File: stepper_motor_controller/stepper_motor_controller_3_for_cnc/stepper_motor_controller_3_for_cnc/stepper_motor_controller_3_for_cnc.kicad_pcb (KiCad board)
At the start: 2 copper layers, 119.4 x 45.7 mm, 44 parts, among them J2 178-009-613R571, U1 74LS74, U11 LM317_TO-220, U3 74LS136

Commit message: centering pcb above origin not below
centering pcb above origin not below
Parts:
- moved R38 144.5 mm to (96.6, -29.9)
- moved R39 144.5 mm to (75.0, -28.6)
- moved R5 144.5 mm to (64.8, -28.6)
- moved R70 144.5 mm to (64.8, -3.23)
- moved R72 144.5 mm to (75.0, -3.23)
- moved U10 144.5 mm to (54.7, -7.05)
- moved U9 144.5 mm to (62.3, -24.8)
- moved J2 144.5 mm to (121.9, -15.9)
- moved R17 144.5 mm to (101.7, -18.5)
- moved R18 144.5 mm to (89.0, -21.0)
- moved R37 144.5 mm to (91.5, -27.4)
- moved R44 144.5 mm to (42.0, -28.6)
- moved R47 144.5 mm to (24.2, -28.4)
- moved R49 144.5 mm to (31.8, -3.23)
- moved R60 144.5 mm to (31.8, -28.6)
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
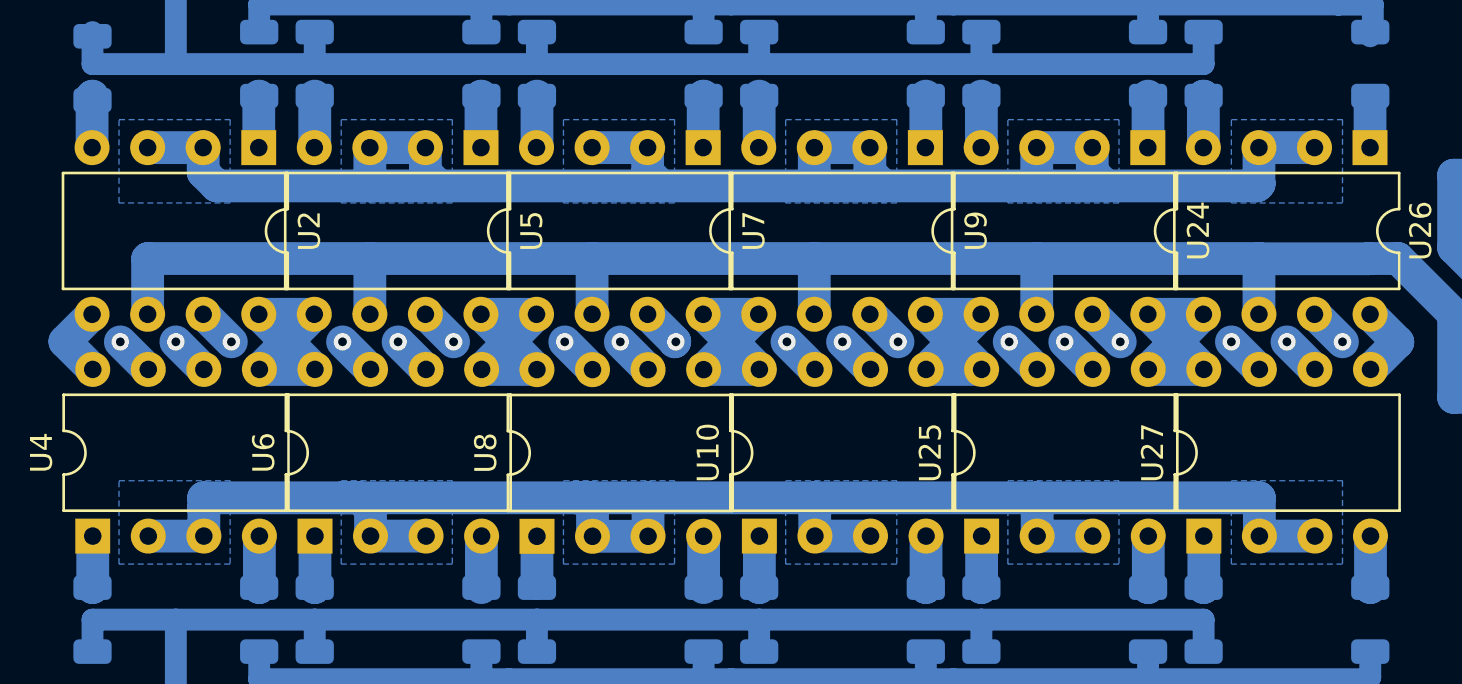
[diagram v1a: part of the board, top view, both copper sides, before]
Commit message: pcb errors
pcb errors
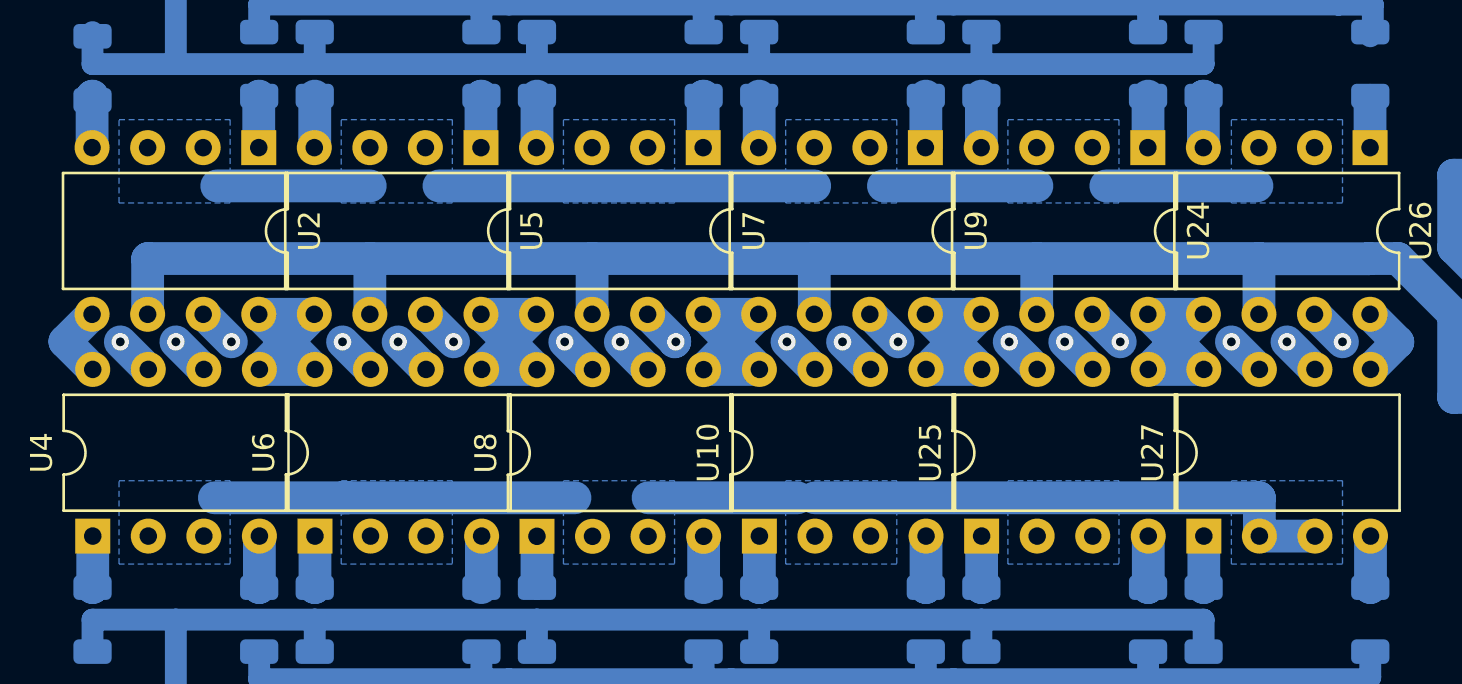
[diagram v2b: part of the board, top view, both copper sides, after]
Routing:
- net VCC: track 207.9 -> 136.8 mm
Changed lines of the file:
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@@
   (segment (start 49.5938 -14.66) (end 48.3238 -15.93) (width 1.5) (layer "B.Cu") (net 16))
   (via (at 99.9338 -35.11) (size 3) (drill 2.4) (layers "F.Cu" "B.Cu") (free) (net 17))
-  (segment (start 49.5938 -7.04) (end 47.0538 -7.04) (width 1.5) (layer "B.Cu") (net 17))
   (segment (start 124.5488 -26.065) (end 114.3888 -26.065) (width 0.5) (layer "B.Cu") (net 17))
-  (segment (start 49.5938 -8.8) (end 57.2138 -8.8) (width 1.5) (layer "B.Cu") (net 17))
-  (segment (start 46.2538 -8.8) (end 49.5938 -8.8) (width 1.5) (layer "B.Cu") (net 17))
   (segment (start 104.8388 -29.9) (end 104.8388 -30.205) (width 1.5) (layer "B.Cu") (net 17))
   (segment (start 127.2938 -18.7) (end 128.3338 -19.74) (width 0.5) (layer "B.Cu") (net 17))
-  (segment (start 47.0338 -24.81) (end 49.5738 -24.81) (width 1.5) (layer "B.Cu") (net 17))
-  (segment (start 77.5338 -23.160382) (end 77.433418 -23.06) (width 1.5) (layer "B.Cu") (net 17))
-  (segment (start 67.3738 -8.8) (end 67.3838 -8.79) (width 1.5) (layer "B.Cu") (net 17))
   (segment (start 77.5338 -8.8) (end 77.5438 -8.79) (width 1.5) (layer "B.Cu") (net 17))
-  (segment (start 57.1938 -24.81) (end 59.7338 -24.81) (width 1.5) (layer "B.Cu") (net 17))
-  (segment (start 36.8738 -23.08) (end 36.8938 -23.06) (width 1.5) (layer "B.Cu") (net 17))
-  (segment (start 40.03243 -23.06) (end 39.4138 -23.67863) (width 1.5) (layer "B.Cu") (net 17))
-  (segment (start 39.4438 -7.05) (end 36.9038 -7.05) (width 1.5) (layer "B.Cu") (net 17))
-  (segment (start 77.5238 -23.170382) (end 77.5338 -23.160382) (width 1.5) (layer "B.Cu") (net 17))
-  (segment (start 36.8738 -24.81) (end 39.4138 -24.81) (width 1.5) (layer "B.Cu") (net 17))
-  (segment (start 26.7138 -24.81) (end 29.2538 -24.81) (width 1.5) (layer "B.Cu") (net 17))
-  (segment (start 39.4138 -23.67863) (end 39.4138 -24.81) (width 1.5) (layer "B.Cu") (net 17))
-  (segment (start 29.2738 -8.31) (end 29.2738 -8.8) (width 1.5) (layer "B.Cu") (net 17))
-  (segment (start 67.3638 -23.07) (end 67.3738 -23.06) (width 1.5) (layer "B.Cu") (net 17))
-  (segment (start 36.4038 -8.8) (end 36.9038 -8.3) (width 1.5) (layer "B.Cu") (net 17))
-  (segment (start 49.5938 -7.04) (end 49.5938 -8.8) (width 1.5) (layer "B.Cu") (net 17))
+  (segment (start 35.6238 -8.8) (end 35.9138 -8.8) (width 1.5) (layer "B.Cu") (net 17))
+  (segment (start 29.7638 -8.8) (end 35.6238 -8.8) (width 1.5) (layer "B.Cu") (net 17))
   (segment (start 36.8938 -23.06) (end 29.87243 -23.06) (width 1.5) (layer "B.Cu") (net 17))
-  (segment (start 29.87243 -23.06) (end 29.2538 -23.67863) (width 1.5) (layer "B.Cu") (net 17))
-  (segment (start 59.7638 -7.05) (end 57.2238 -7.05) (width 1.5) (layer "B.Cu") (net 17))
   (segment (start 104.8388 -30.205) (end 99.9338 -35.11) (width 1.5) (layer "B.Cu") (net 17))
-  (segment (start 57.2138 -7.06) (end 57.2238 -7.05) (width 1.5) (layer "B.Cu") (net 17))
   (segment (start 77.5438 -8.79) (end 77.5438 -7.05) (width 1.5) (layer "B.Cu") (net 17))
-  (segment (start 29.2738 -8.8) (end 35.6238 -8.8) (width 1.5) (layer "B.Cu") (net 17))
-  (segment (start 60.35243 -23.06) (end 59.7338 -23.67863) (width 1.5) (layer "B.Cu") (net 17))
-  (segment (start 40.03243 -23.06) (end 36.8938 -23.06) (width 1.5) (layer "B.Cu") (net 17))
   (segment (start 80.0838 -7.05) (end 77.5438 -7.05) (width 1.5) (layer "B.Cu") (net 17))
-  (segment (start 49.5738 -23.67863) (end 49.5738 -24.81) (width 1.5) (layer "B.Cu") (net 17))
-  (segment (start 77.5238 -24.81) (end 77.5238 -23.170382) (width 1.5) (layer "B.Cu") (net 17))
   (segment (start 57.2138 -23.06) (end 50.19243 -23.06) (width 1.5) (layer "B.Cu") (net 17))
-  (segment (start 70.52243 -23.06) (end 67.3738 -23.06) (width 1.5) (layer "B.Cu") (net 17))
-  (segment (start 69.9238 -7.05) (end 67.3838 -7.05) (width 1.5) (layer "B.Cu") (net 17))
-  (segment (start 29.2838 -8.3) (end 29.2738 -8.31) (width 1.5) (layer "B.Cu") (net 17))
-  (segment (start 46.2538 -8.8) (end 47.0538 -8.8) (width 1.5) (layer "B.Cu") (net 17))
-  (segment (start 67.3638 -24.81) (end 69.9038 -24.81) (width 1.5) (layer "B.Cu") (net 17))
-  (segment (start 57.1938 -24.81) (end 57.1938 -23.08) (width 1.5) (layer "B.Cu") (net 17))
+  (segment (start 49.5938 -8.8) (end 56.4338 -8.8) (width 1.5) (layer "B.Cu") (net 17))
   (segment (start 114.3888 -26.065) (end 111.8238 -28.63) (width 0.5) (layer "B.Cu") (net 17))
-  (segment (start 36.8738 -24.81) (end 36.8738 -23.08) (width 1.5) (layer "B.Cu") (net 17))
   (segment (start 116.3488 -18.7) (end 123.0988 -18.7) (width 0.5) (layer "B.Cu") (net 17))
   (segment (start 57.2138 -8.8) (end 77.5338 -8.8) (width 1.5) (layer "B.Cu") (net 17))
-  (segment (start 35.6238 -8.8) (end 36.4038 -8.8) (width 1.5) (layer "B.Cu") (net 17))
-  (segment (start 57.1938 -23.08) (end 57.2138 -23.06) (width 1.5) (layer "B.Cu") (net 17))
-  (segment (start 69.9038 -23.67863) (end 69.9038 -24.81) (width 1.5) (layer "B.Cu") (net 17))
-  (segment (start 70.52243 -23.06) (end 69.9038 -23.67863) (width 1.5) (layer "B.Cu") (net 17))
   (segment (start 77.433418 -23.06) (end 70.52243 -23.06) (width 1.5) (layer "B.Cu") (net 17))
   (segment (start 67.3738 -23.06) (end 60.35243 -23.06) (width 1.5) (layer "B.Cu") (net 17))
-  (segment (start 50.19243 -23.06) (end 49.5738 -23.67863) (width 1.5) (layer "B.Cu") (net 17))
-  (segment (start 29.2838 -7.05) (end 29.2838 -8.3) (width 1.5) (layer "B.Cu") (net 17))
-  (segment (start 67.3638 -24.81) (end 67.3638 -23.07) (width 1.5) (layer "B.Cu") (net 17))
-  (segment (start 29.2838 -7.05) (end 26.7438 -7.05) (width 1.5) (layer "B.Cu") (net 17))
-  (segment (start 59.7338 -23.67863) (end 59.7338 -24.81) (width 1.5) (layer "B.Cu") (net 17))
-  (segment (start 67.3838 -8.79) (end 67.3838 -7.05) (width 1.5) (layer "B.Cu") (net 17))
   (segment (start 35.6238 -8.8) (end 46.2538 -8.8) (width 1.5) (layer "B.Cu") (net 17))
   (segment (start 123.0988 -18.7) (end 127.2938 -18.7) (width 0.5) (layer "B.Cu") (net 17))
-  (segment (start 77.5238 -24.81) (end 80.0638 -24.81) (width 1.5) (layer "B.Cu") (net 17))
   (segment (start 50.19243 -23.06) (end 40.03243 -23.06) (width 1.5) (layer "B.Cu") (net 17))
   (segment (start 128.3338 -19.74) (end 128.3338 -22.28) (width 0.5) (layer "B.Cu") (net 17))
   (segment (start 106.1088 -28.63) (end 104.8388 -29.9) (width 0.5) (layer "B.Cu") (net 17))
-  (segment (start 57.2138 -8.8) (end 57.2138 -7.06) (width 1.5) (layer "B.Cu") (net 17))
   (segment (start 104.8388 -28.32) (end 104.8388 -29.9) (width 1.5) (layer "B.Cu") (net 17))
-  (segment (start 47.0538 -8.8) (end 47.0538 -7.04) (width 1.5) (layer "B.Cu") (net 17))
-  (segment (start 60.35243 -23.06) (end 57.2138 -23.06) (width 1.5) (layer "B.Cu") (net 17))
-  (segment (start 36.9038 -8.3) (end 36.9038 -7.05) (width 1.5) (layer "B.Cu") (net 17))
-  (segment (start 29.2538 -23.67863) (end 29.2538 -24.81) (width 1.5) (layer "B.Cu") (net 17))
   (segment (start 111.8238 -28.63) (end 106.1088 -28.63) (width 0.5) (layer "B.Cu") (net 17))
   (segment (start 128.3338 -22.28) (end 124.5488 -26.065) (width 0.5) (layer "B.Cu") (net 17))
@@
     (priority 1)
     (connect_pads yes (clearance 0.5))
-    (min_thickness 0.25) (filled_areas_thickness no)
-    (fill yes (thermal_gap 0.5) (thermal_bridge_width 0.5))
-    (polygon
-      (pts
+    (min_thickness 1.5) (filled_areas_thickness no)
+    (fill yes (thermal_gap 0.5) (thermal_bridge_width 1.5))
+    (polygon
+      (pts

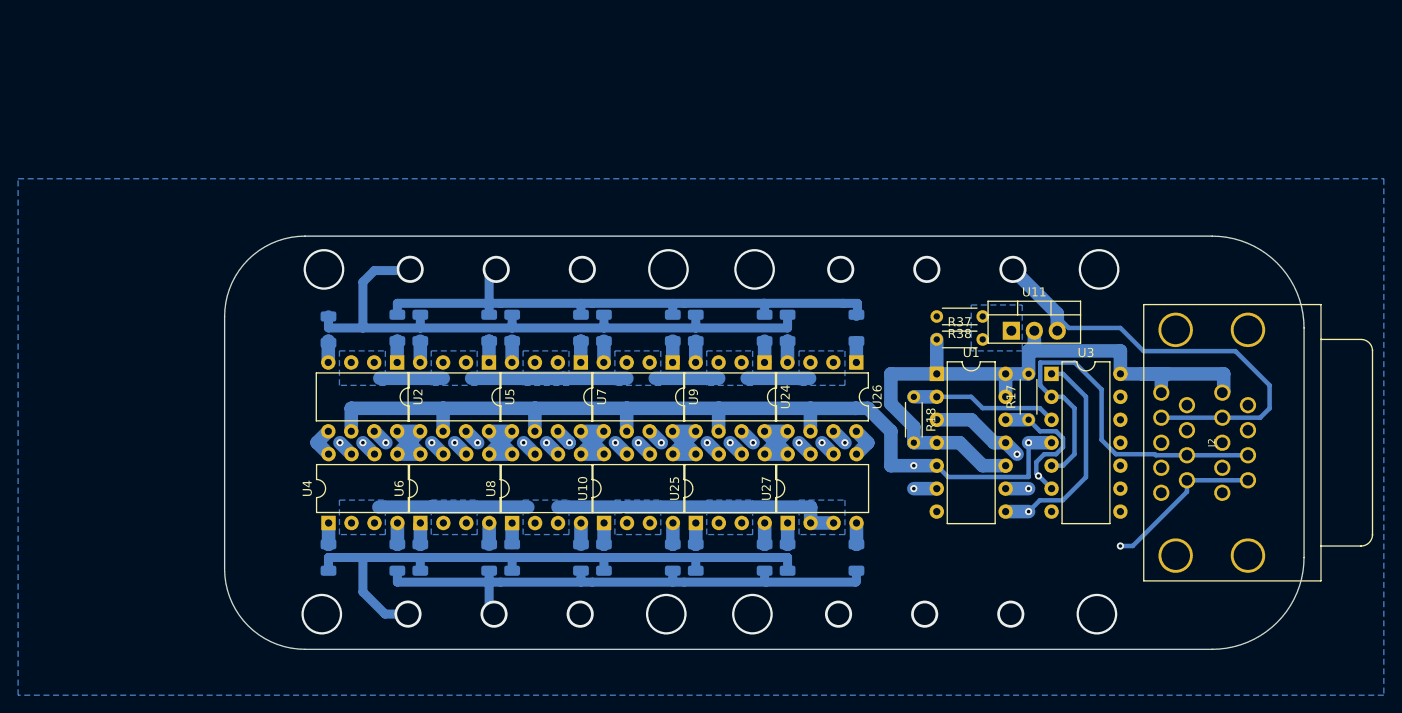
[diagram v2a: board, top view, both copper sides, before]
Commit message: moving board
moving board
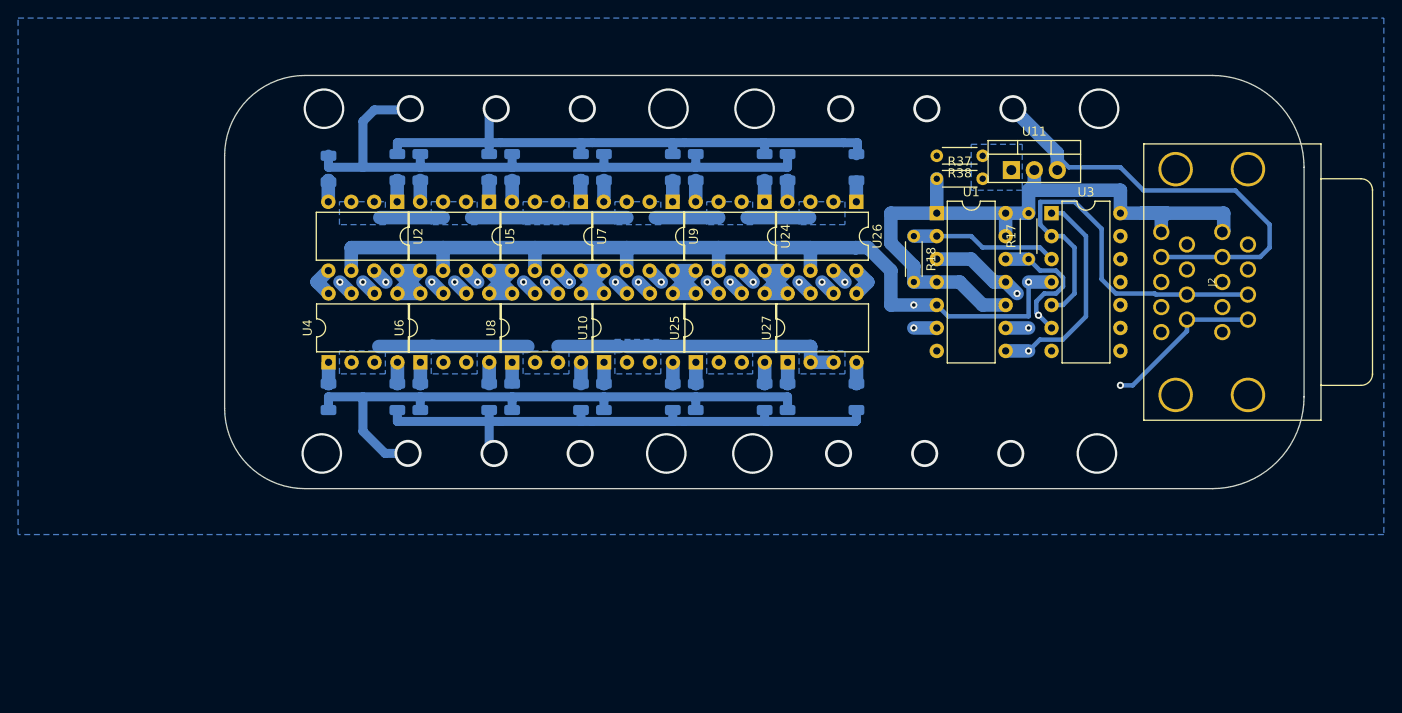
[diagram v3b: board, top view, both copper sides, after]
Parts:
- moved U2 17.8 mm to (31.8, -42.6)
- moved U24 17.8 mm to (72.4, -42.6)
- moved U26 17.8 mm to (82.6, -42.6)
- moved U5 17.8 mm to (42.0, -42.6)
- moved U7 17.8 mm to (52.1, -42.6)
- moved U9 17.8 mm to (62.3, -42.6)
- moved J2 17.8 mm to (121.9, -33.7)
- moved R12 17.8 mm to (54.7, -21.0)
- moved R17 17.8 mm to (101.7, -36.2)
- moved R3 17.8 mm to (82.6, -21.0)
- moved R37 17.8 mm to (91.5, -45.1)
- moved R38 17.8 mm to (96.6, -47.7)
- moved R46 17.8 mm to (34.4, -21.0)
- moved R47 17.8 mm to (24.2, -46.2)
- moved R49 17.8 mm to (31.8, -21.0)
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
